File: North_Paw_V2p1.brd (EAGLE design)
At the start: 67.5 x 44.5 mm, 19 parts, among them Q2 8MHz

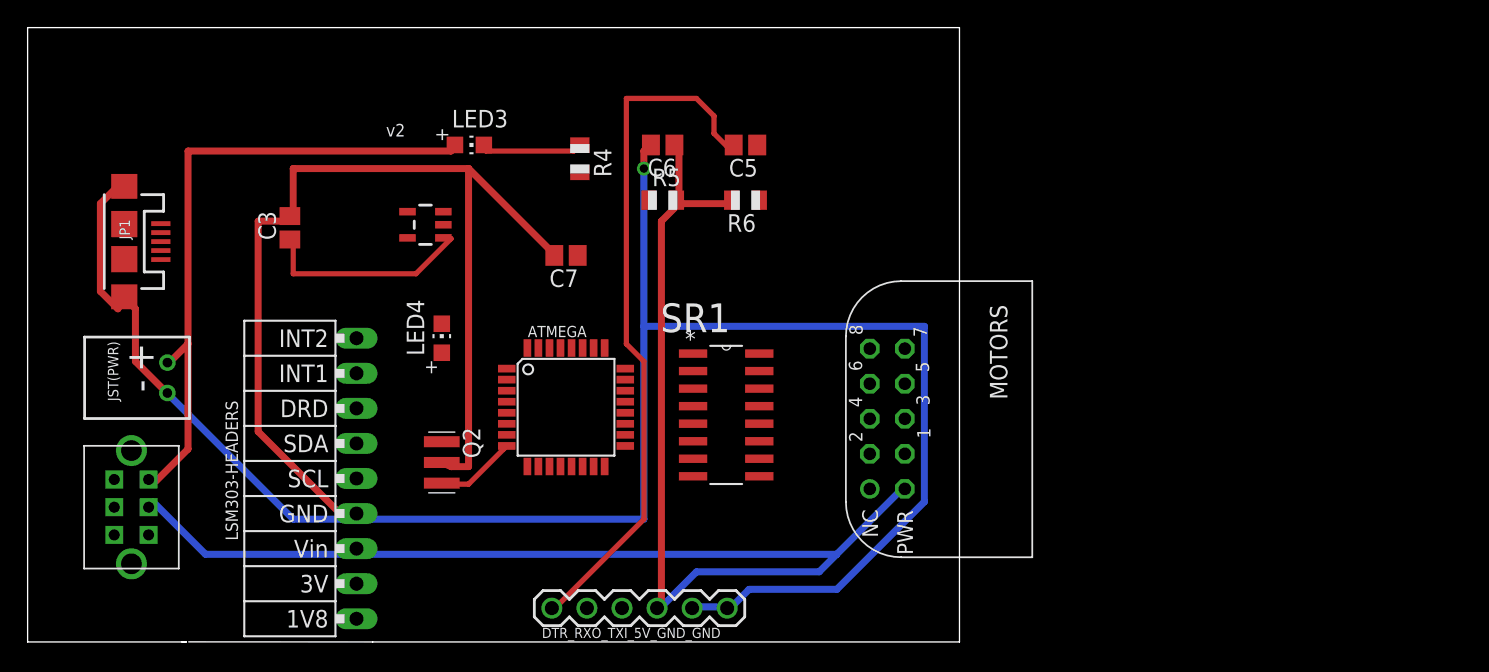
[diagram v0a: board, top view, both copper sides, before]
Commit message: Initial checkin of TopoR
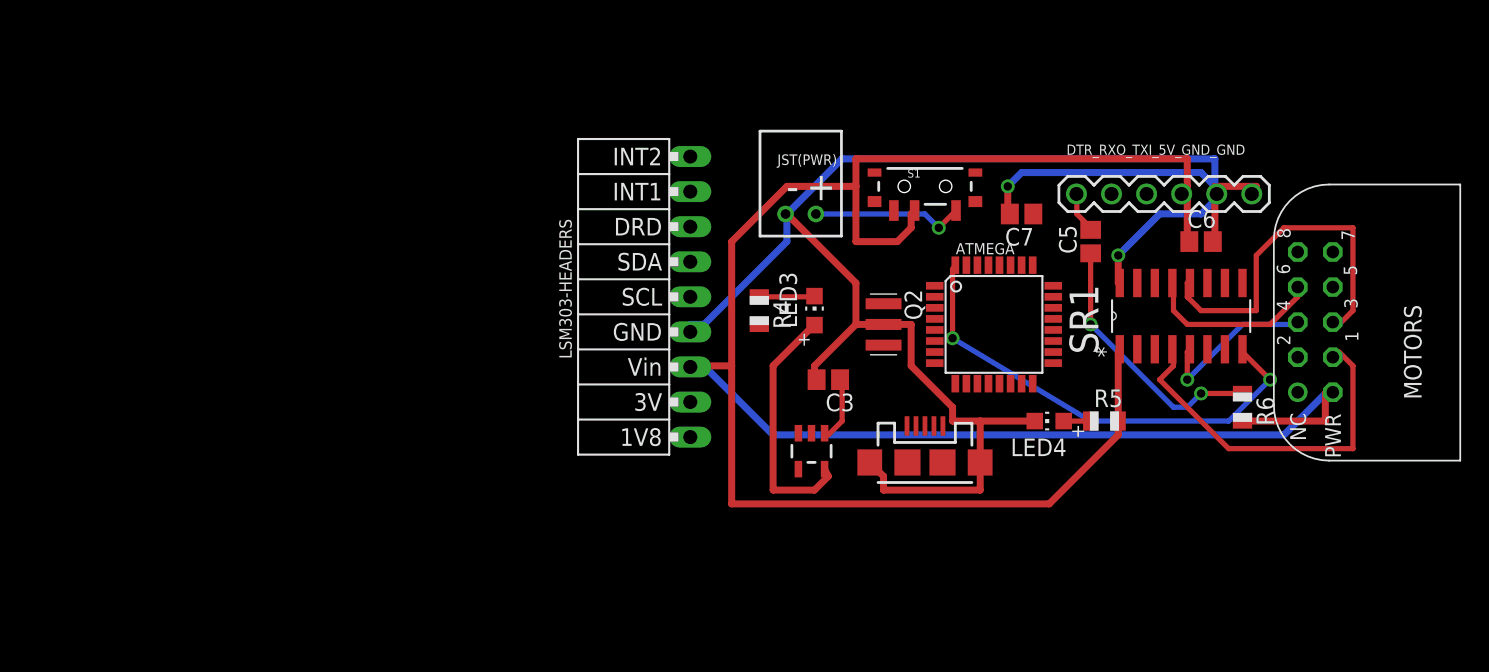
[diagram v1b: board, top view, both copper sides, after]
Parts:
- removed SWITCH: OS202011MA0QS1, OS202011MA0QS1:OS202011MA0QS1
- added S1: (no value), SparkFun-Electromechanical:SWITCH-SPST-SMD-A
- moved JP1 60.2 mm to (61.0, 13.0), turned to 0 degrees
- moved FTDI 48.4 mm to (72.0, 32.5)
- moved JST(PWR) 47.4 mm to (52.0, 31.0), turned to 180 degrees
- moved LED4 44.4 mm to (70.0, 16.0), turned to 90 degrees
- moved C3 40.5 mm to (54.0, 19.0), turned to 180 degrees
- moved C6 39.6 mm to (81.0, 29.0), turned to 0 degrees
- moved R6 39.0 mm to (84.0, 17.0), turned to 270 degrees
- moved SR1 37.7 mm to (84.0, 26.0), turned to 90 degrees
- moved R5 35.8 mm to (74.0, 16.0)
- moved Q2 33.5 mm to (58.0, 23.0)
- moved C7 33.1 mm to (68.0, 31.0)
- moved CHARGER 32.4 mm to (52.8, 13.8), turned to 180 degrees
- moved MOTORS 31.8 mm to (94.3, 23.1)
- moved ATMEGA 31.6 mm to (66.0, 23.0)
- moved LED3 27.7 mm to (53.0, 24.0), turned to 0 degrees
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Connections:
- removed net 1: SWITCH.1
- removed net 2: SWITCH.2
- removed net 3: SWITCH.3
- removed net 4: SWITCH.4
- new net N$4: JST(PWR).PWR, S1.3
- net 3.3V: now also S1.2; no longer SWITCH.5
- net BATT: no longer JST(PWR).PWR, SWITCH.6
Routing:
- net GND: track 216.9 -> 132.6 mm, vias 1 -> 2
- net 3.3V: track 112.8 -> 169.7 mm
- net DTR: track 50.7 -> 3.02 mm
- net D2: track 0.00 -> 34.3 mm, vias 0 -> 2
- net BATT: track 47.3 -> 18.3 mm
- net M2: track 0.00 -> 26.7 mm
- net M4: track 0.00 -> 26.3 mm
- net RESET: track 0.00 -> 19.0 mm, vias 0 -> 2
- net M5: track 0.00 -> 13.0 mm
- net M3: track 0.00 -> 12.1 mm, vias 0 -> 1
- net N$4: track 0.00 -> 11.2 mm, vias 0 -> 1
- net USB_VIN: track 15.8 -> 4.86 mm
- net N$2: track 5.86 -> 0.00 mm
- net N$8: track 7.44 -> 4.05 mm
- net A0: track 0.00 -> 2.00 mm
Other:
- board outline removed
- board text removed: "X:/Dropbox/Sensebridge/eagle/bmps/North_Paw_JUST_NP.bmp"
- board text removed: "v2"
